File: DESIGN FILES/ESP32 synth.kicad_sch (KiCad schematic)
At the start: 4 parts

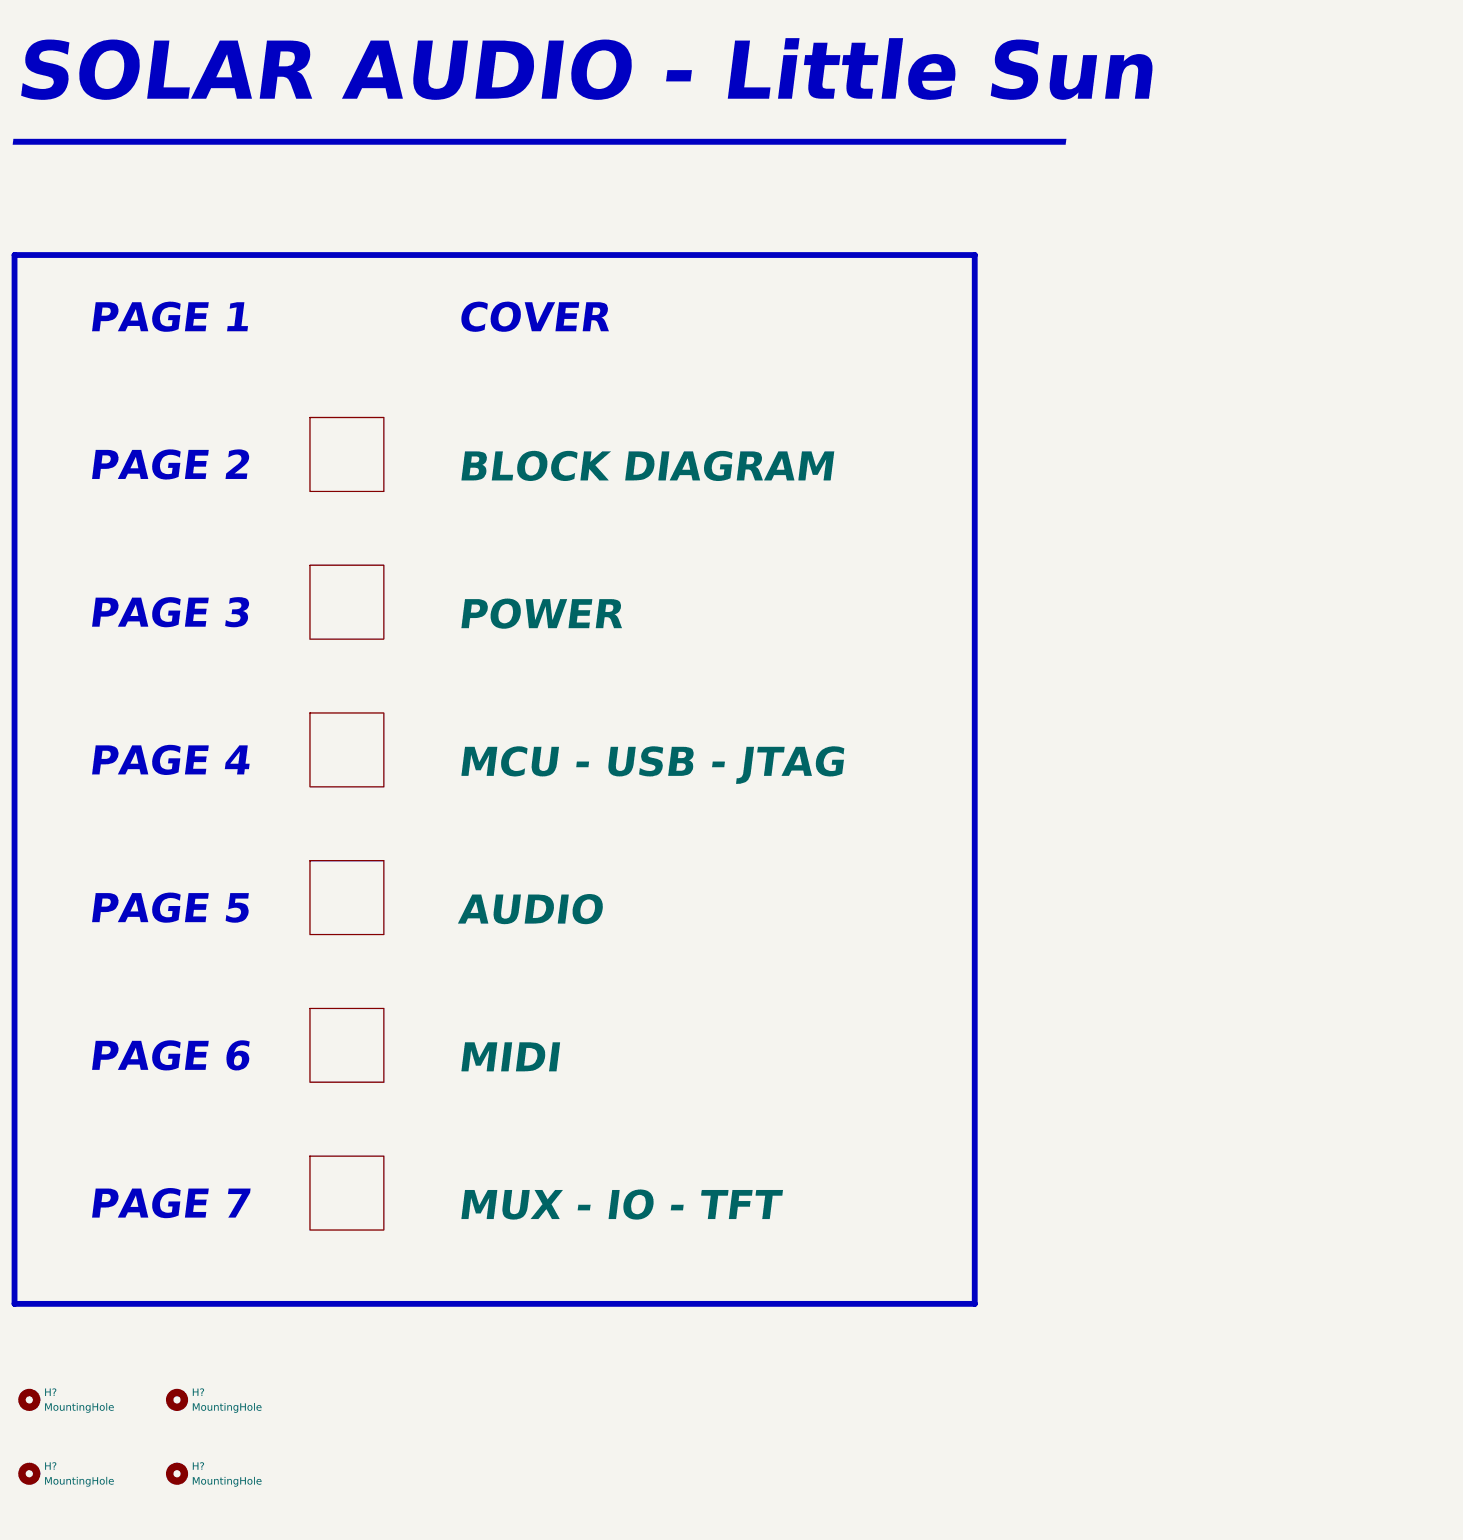
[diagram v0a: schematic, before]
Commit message: updates
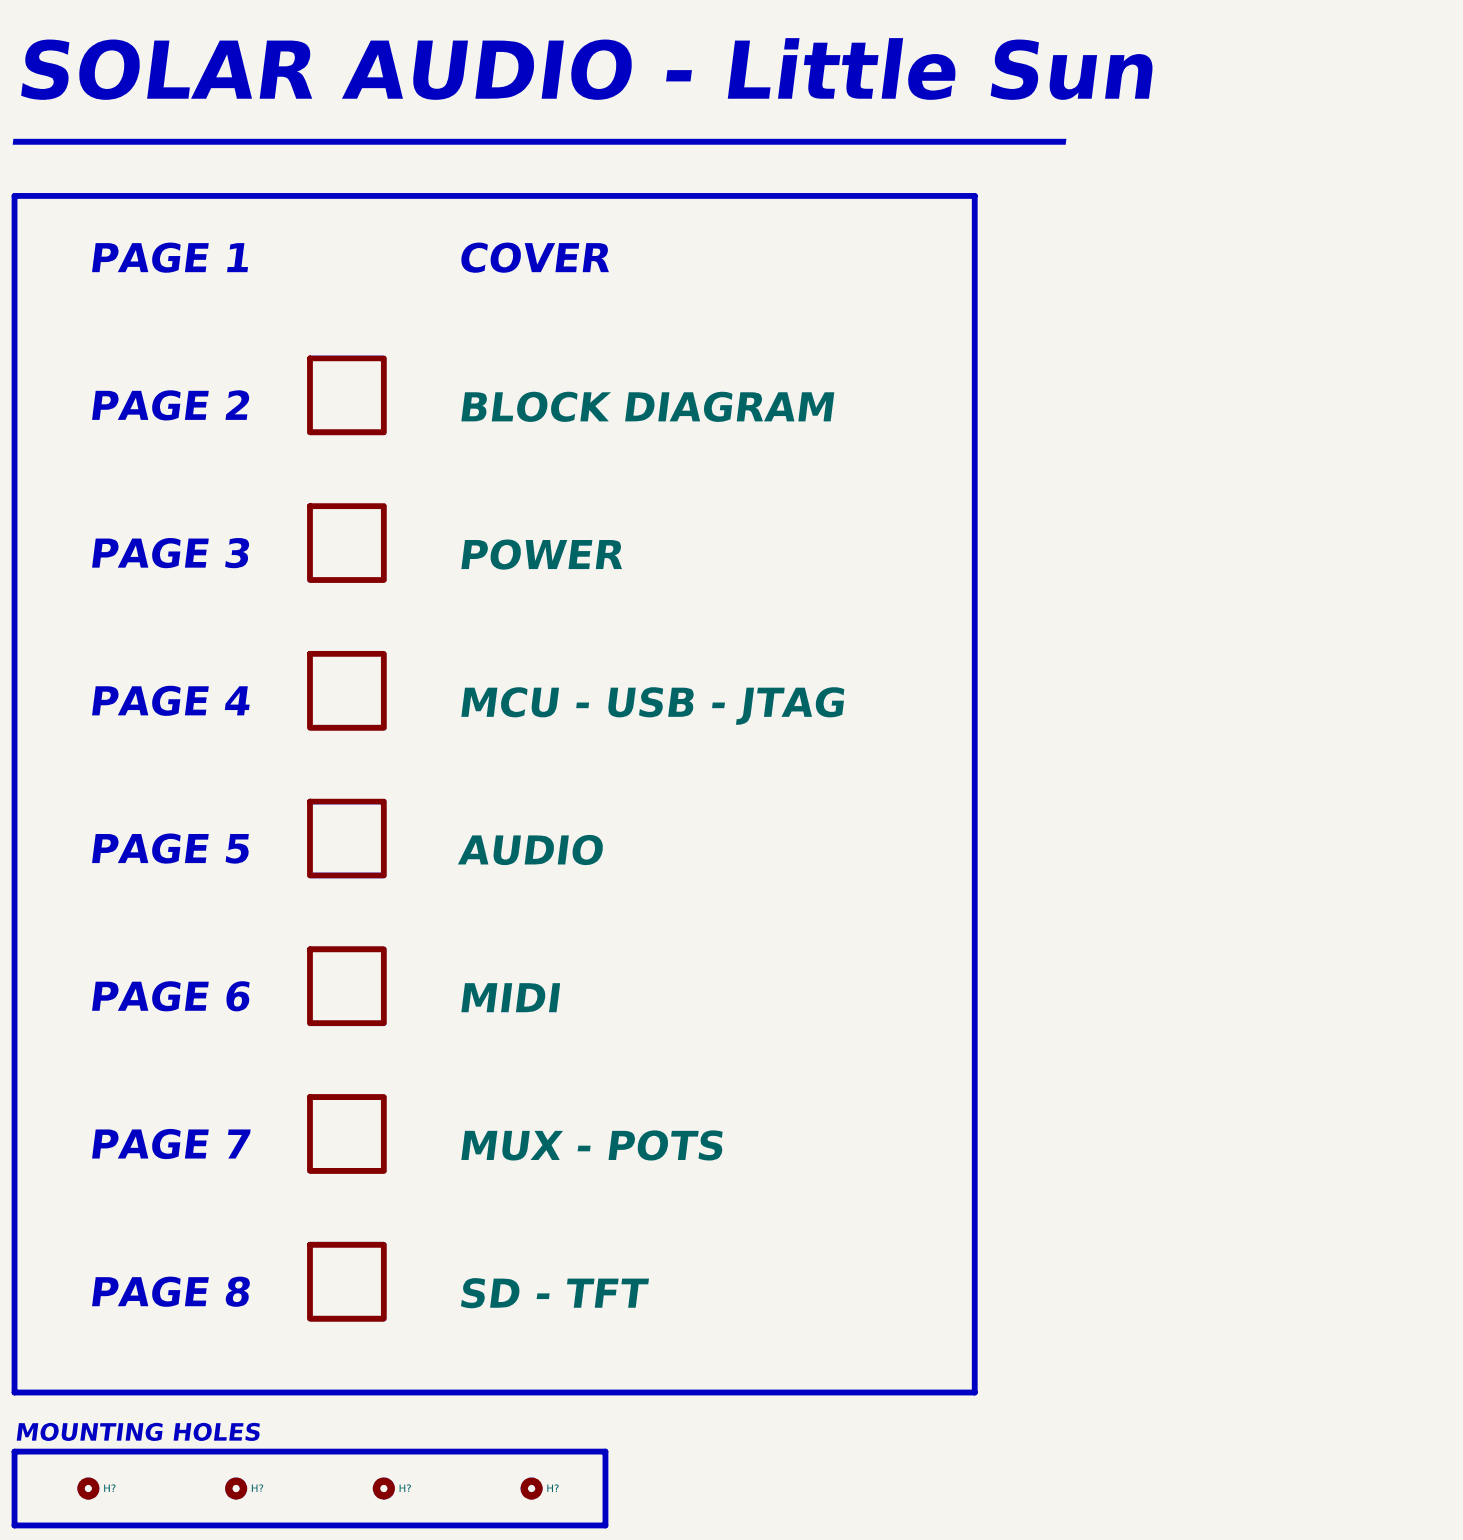
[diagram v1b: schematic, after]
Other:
- sheet MUX - IO - TFT renamed MUX - POTS
- added sheet SD - TFT (sd_tft.kicad_sch)
- note added: "MOUNTING HOLES"
- note added: "PAGE 8"
- moved on the sheet: H?
